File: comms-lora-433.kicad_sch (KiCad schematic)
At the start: 13 parts, among them J4 Conn_Coaxial_Small, U5 RFM69W

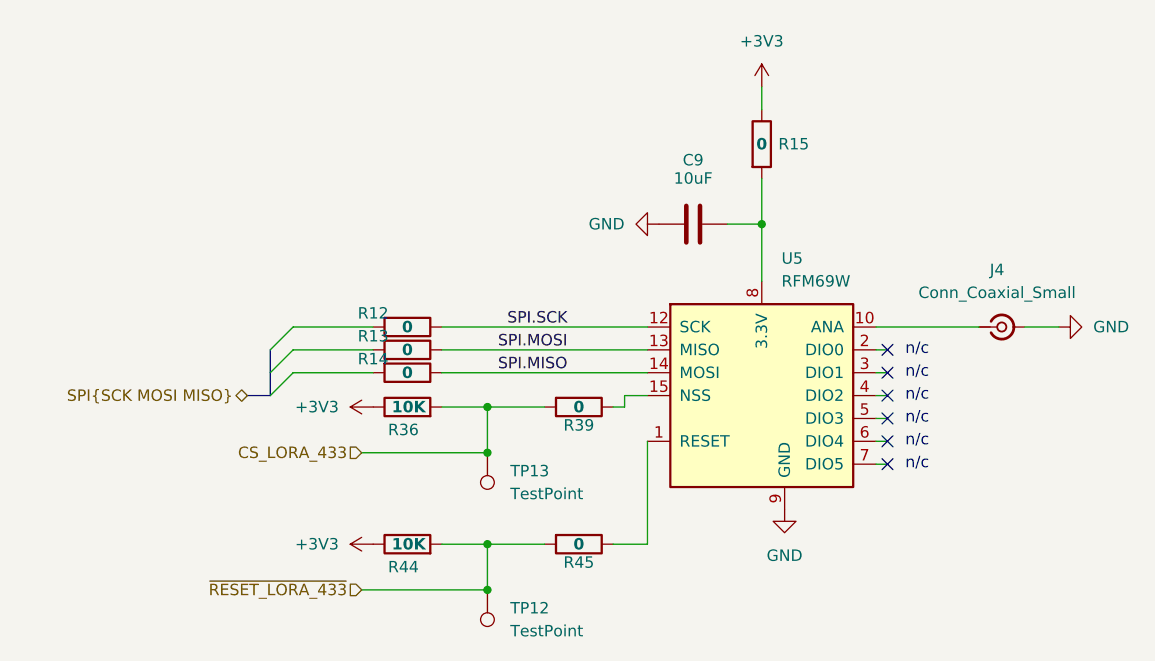
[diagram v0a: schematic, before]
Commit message: Fixing lots of ERC errors
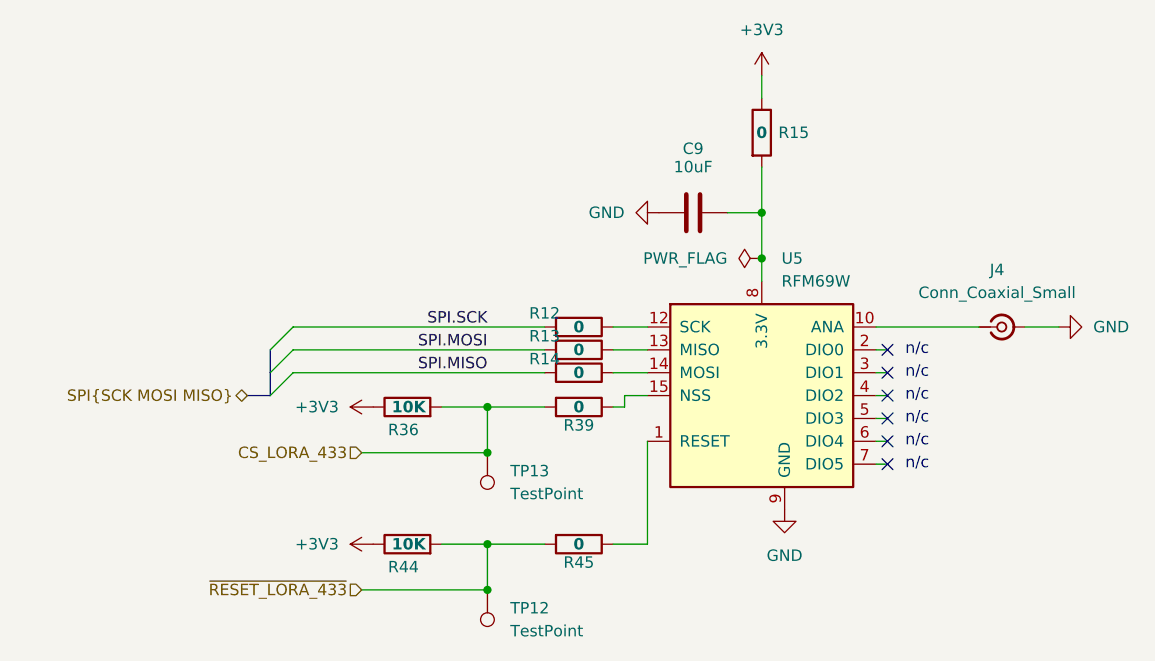
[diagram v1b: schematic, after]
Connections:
- net SPI.MISO: now also R14.2; no longer R14.1, U5.14 (MOSI)
- net SPI.MOSI: now also R13.2; no longer R13.1, U5.13 (MISO)
- net SPI.SCK: now also R12.2; no longer R12.1, U5.12 (SCK)
- new net: R12.1, U5.12 (SCK)
- new net: R13.1, U5.13 (MISO)
- new net: R14.1, U5.14 (MOSI)
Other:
- moved on the sheet: C9, R12, R13, R14, R15
